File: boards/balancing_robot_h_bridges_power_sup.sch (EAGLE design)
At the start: 19 parts

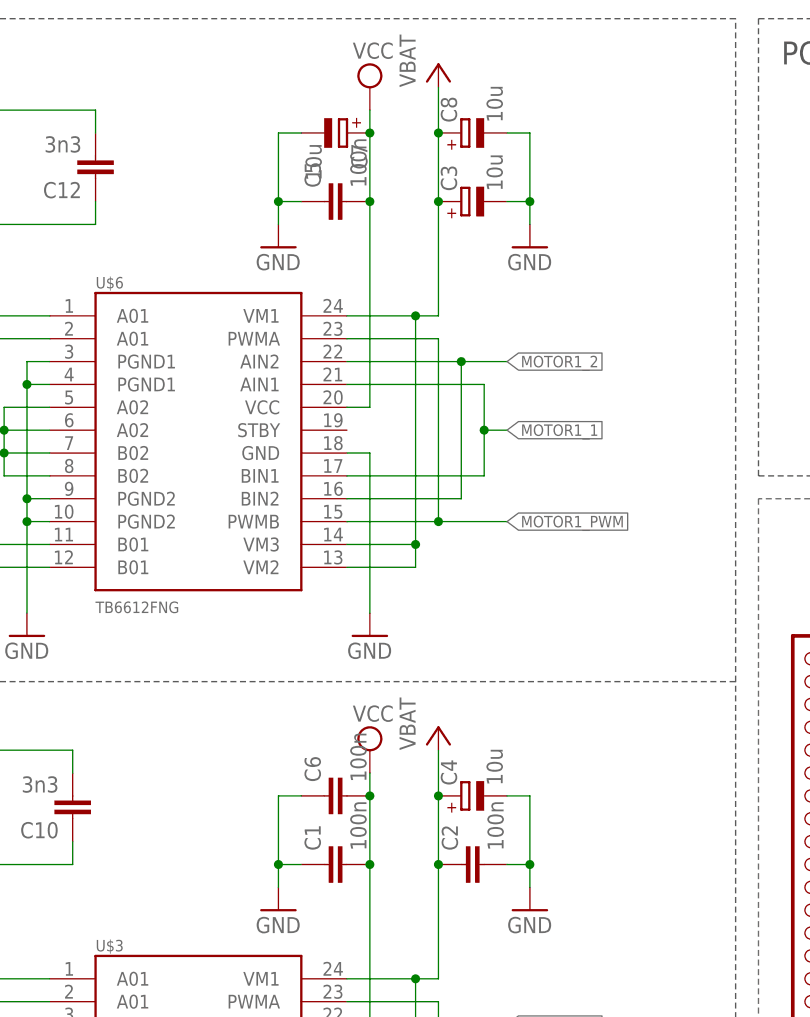
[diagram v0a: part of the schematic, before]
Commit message: updated bridge board
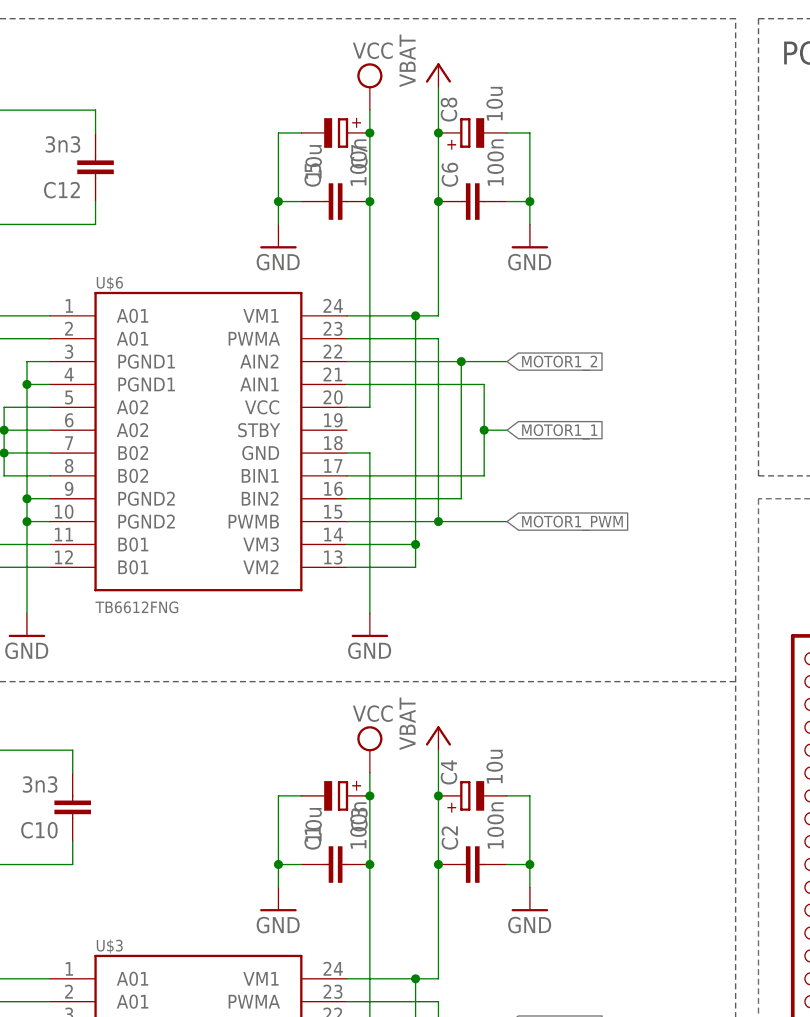
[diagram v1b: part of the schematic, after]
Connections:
- removed net N$5: U$3.PGND1@3, U$3.PGND1@4, U$3.PGND2@10, U$3.PGND2@9, U$6.PGND1@3, U$6.PGND1@4, U$6.PGND2@10, U$6.PGND2@9
- net GND: now also C6.2, U$3.PGND1@3, U$3.PGND1@4, U$3.PGND2@10, U$3.PGND2@9, U$6.PGND1@3, U$6.PGND1@4, U$6.PGND2@10, U$6.PGND2@9; no longer C6.1
- net VCC: now also C6.1; no longer C6.2
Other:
- moved on the sheet: C3, C6
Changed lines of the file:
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@@
 <part name="SUPPLY1" library="supply2" deviceset="VCC" device=""/>
 <part name="VAABT" library="supply1" deviceset="VCC" device="" value="VBAT"/>
-<part name="GND4" library="supply1" deviceset="GND" device=""/>
 <part name="GND5" library="supply1" deviceset="GND" device=""/>
 <part name="SUPPLY3" library="supply2" deviceset="VCC" device=""/>
@@
 <part name="GND7" library="supply1" deviceset="GND" device=""/>
 <part name="U$6" library="SparkFun-PowerIC" deviceset="TB6612FNG" device="" value="TB6612FNG"/>
-<part name="GND8" library="supply1" deviceset="GND" device=""/>
 <part name="GND9" library="supply1" deviceset="GND" device=""/>
 <part name="SUPPLY4" library="supply2" deviceset="VCC" device=""/>
-<part name="VAABT2" library="supply1" deviceset="VCC" device="" value="VBAT"/>
+<part name="VBAT" library="supply1" deviceset="VCC" device="" value="VBAT"/>
 <part name="C5" library="rcl" deviceset="C-EU" device="C0603" value="100n"/>
 <part name="GND10" library="supply1" deviceset="GND" device=""/>
@@
 <part name="C8" library="rcl" deviceset="CPOL-EU" device="153CLV-0405" value="10u"/>
 <part name="JP1" library="pinhead" deviceset="PINHD-1X24" device=""/>
-<part name="C3" library="rcl" deviceset="CPOL-EU" device="153CLV-0405" value="10u"/>
 <part name="C7" library="rcl" deviceset="CPOL-EU" device="153CLV-0405" value="10u"/>
-<part name="C6" library="rcl" deviceset="C-EU" device="C0603" value="100n"/>
 <part name="GND3" library="supply1" deviceset="GND" device=""/>
 <part name="VAABT3" library="supply1" deviceset="VCC" device="" value="VBAT"/>
+<part name="C3" library="rcl" deviceset="CPOL-EU" device="153CLV-0405" value="10u"/>
+<part name="C6" library="rcl" deviceset="C-EU" device="C0603" value="100n"/>
+<part name="GND8" library="supply1" deviceset="GND" device=""/>
+<part name="GND4" library="supply1" deviceset="GND" device=""/>
 </parts>
 <sheets>
@@
 <instance part="SUPPLY1" gate="G$1" x="195.58" y="134.62"/>
 <instance part="VAABT" gate="VCC" x="132.08" y="137.16"/>
-<instance part="GND4" gate="1" x="25.4" y="5.08"/>
 <instance part="GND5" gate="1" x="63.5" y="5.08"/>
 <instance part="SUPPLY3" gate="G$1" x="63.5" y="66.04"/>
@@
 <instance part="GND7" gate="1" x="81.28" y="48.26"/>
 <instance part="U$6" gate="G$1" x="45.72" y="101.6"/>
-<instance part="GND8" gate="1" x="25.4" y="78.74"/>
 <instance part="GND9" gate="1" x="63.5" y="78.74"/>
 <instance part="SUPPLY4" gate="G$1" x="63.5" y="139.7"/>
-<instance part="VAABT2" gate="VCC" x="71.12" y="142.24"/>
+<instance part="VBAT" gate="VCC" x="71.12" y="142.24"/>
 <instance part="C5" gate="G$1" x="58.42" y="127" rot="R90"/>
 <instance part="GND10" gate="1" x="53.34" y="121.92"/>
@@
 <instance part="C8" gate="G$1" x="73.66" y="134.62" rot="R90"/>
 <instance part="JP1" gate="A" x="111.76" y="45.72" rot="R180"/>
-<instance part="C3" gate="G$1" x="73.66" y="127" rot="R90"/>
 <instance part="C7" gate="G$1" x="60.96" y="134.62" rot="R270"/>
-<instance part="C6" gate="G$1" x="58.42" y="60.96" rot="R90"/>
 <instance part="GND3" gate="1" x="127" y="10.16"/>
 <instance part="VAABT3" gate="VCC" x="152.4" y="27.94"/>
+<instance part="C3" gate="G$1" x="60.96" y="60.96" rot="R270"/>
+<instance part="C6" gate="G$1" x="73.66" y="127" rot="R90"/>
+<instance part="GND8" gate="1" x="25.4" y="78.74"/>
+<instance part="GND4" gate="1" x="25.4" y="5.08"/>
 </instances>
 <busses>
@@
 <junction x="53.34" y="53.34"/>
 <pinref part="GND6" gate="1" pin="GND"/>
-<pinref part="C6" gate="G$1" pin="1"/>
+<pinref part="C3" gate="G$1" pin="-"/>
 </segment>
 <segment>
@@
 <pinref part="GND11" gate="1" pin="GND"/>
 <pinref part="C8" gate="G$1" pin="-"/>
-<pinref part="C3" gate="G$1" pin="-"/>
+<pinref part="C6" gate="G$1" pin="2"/>
 </segment>
 <segment>
@@
 <junction x="124.46" y="27.94"/>
 <pinref part="GND3" gate="1" pin="GND"/>
+</segment>
+<segment>
+<pinref part="U$6" gate="G$1" pin="PGND1@3"/>
+<wire x1="27.94" y1="109.22" x2="25.4" y2="109.22" width="0.1524" layer="91"/>
+<wire x1="25.4" y1="109.22" x2="25.4" y2="106.68" width="0.1524" layer="91"/>
+<pinref part="U$6" gate="G$1" pin="PGND2@10"/>
+<wire x1="25.4" y1="106.68" x2="25.4" y2="93.98" width="0.1524" layer="91"/>
+<wire x1="25.4" y1="93.98" x2="25.4" y2="91.44" width="0.1524" layer="91"/>
+<wire x1="25.4" y1="91.44" x2="25.4" y2="81.28" width="0.1524" layer="91"/>
+<wire x1="27.94" y1="91.44" x2="25.4" y2="91.44" width="0.1524" layer="91"/>
+<junction x="25.4" y="91.44"/>
+<pinref part="U$6" gate="G$1" pin="PGND2@9"/>
+<wire x1="27.94" y1="93.98" x2="25.4" y2="93.98" width="0.1524" layer="91"/>
+<junction x="25.4" y="93.98"/>
+<pinref part="U$6" gate="G$1" pin="PGND1@4"/>
+<wire x1="27.94" y1="106.68" x2="25.4" y2="106.68" width="0.1524" layer="91"/>
+<junction x="25.4" y="106.68"/>
+<pinref part="GND8" gate="1" pin="GND"/>
+</segment>
+<segment>
+<pinref part="U$3" gate="G$1" pin="PGND1@3"/>
+<wire x1="27.94" y1="35.56" x2="25.4" y2="35.56" width="0.1524" layer="91"/>
+<wire x1="25.4" y1="35.56" x2="25.4" y2="33.02" width="0.1524" layer="91"/>
+<pinref part="U$3" gate="G$1" pin="PGND2@10"/>
+<wire x1="25.4" y1="33.02" x2="25.4" y2="20.32" width="0.1524" layer="91"/>
+<wire x1="25.4" y1="20.32" x2="25.4" y2="17.78" width="0.1524" layer="91"/>
+<wire x1="25.4" y1="17.78" x2="25.4" y2="7.62" width="0.1524" layer="91"/>
+<wire x1="27.94" y1="17.78" x2="25.4" y2="17.78" width="0.1524" layer="91"/>
+<junction x="25.4" y="17.78"/>
+<pinref part="U$3" gate="G$1" pin="PGND2@9"/>
+<wire x1="27.94" y1="20.32" x2="25.4" y2="20.32" width="0.1524" layer="91"/>
+<junction x="25.4" y="20.32"/>
+<pinref part="U$3" gate="G$1" pin="PGND1@4"/>
+<wire x1="27.94" y1="33.02" x2="25.4" y2="33.02" width="0.1524" layer="91"/>
+<junction x="25.4" y="33.02"/>
+<pinref part="GND4" gate="1" pin="GND"/>
 </segment>
 </net>
@@
 <wire x1="63.5" y1="53.34" x2="63.5" y2="60.96" width="0.1524" layer="91"/>
 <junction x="63.5" y="53.34"/>
-<pinref part="C6" gate="G$1" pin="2"/>
+<pinref part="C3" gate="G$1" pin="+"/>
 <wire x1="63.5" y1="60.96" x2="63.5" y2="63.5" width="0.1524" layer="91"/>
 <junction x="63.5" y="60.96"/>
@@
 <wire x1="60.96" y1="88.9" x2="68.58" y2="88.9" width="0.1524" layer="91"/>
 <junction x="68.58" y="88.9"/>
-<pinref part="VAABT2" gate="VCC" pin="VCC"/>
+<pinref part="VBAT" gate="VCC" pin="VCC"/>
 <wire x1="68.58" y1="114.3" x2="71.12" y2="114.3" width="0.1524" layer="91"/>
 <wire x1="71.12" y1="114.3" x2="71.12" y2="127" width="0.1524" layer="91"/>
@@
 <wire x1="71.12" y1="134.62" x2="71.12" y2="139.7" width="0.1524" layer="91"/>
 <junction x="71.12" y="134.62"/>
-<pinref part="C3" gate="G$1" pin="+"/>
+<pinref part="C6" gate="G$1" pin="1"/>
 <junction x="71.12" y="127"/>
 </segment>
@@
 </segment>
 </net>
-<net name="N$5" class="0">
-<segment>
-<pinref part="U$3" gate="G$1" pin="PGND1@3"/>
-<wire x1="27.94" y1="35.56" x2="25.4" y2="35.56" width="0.1524" layer="91"/>
-<wire x1="25.4" y1="35.56" x2="25.4" y2="33.02" width="0.1524" layer="91"/>
-<pinref part="U$3" gate="G$1" pin="PGND2@10"/>
-<wire x1="25.4" y1="33.02" x2="25.4" y2="20.32" width="0.1524" layer="91"/>
-<wire x1="25.4" y1="20.32" x2="25.4" y2="17.78" width="0.1524" layer="91"/>
-<wire x1="25.4" y1="17.78" x2="25.4" y2="7.62" width="0.1524" layer="91"/>
-<wire x1="27.94" y1="17.78" x2="25.4" y2="17.78" width="0.1524" layer="91"/>
-<junction x="25.4" y="17.78"/>
-<pinref part="U$3" gate="G$1" pin="PGND2@9"/>
-<wire x1="27.94" y1="20.32" x2="25.4" y2="20.32" width="0.1524" layer="91"/>
-<junction x="25.4" y="20.32"/>
-<pinref part="U$3" gate="G$1" pin="PGND1@4"/>
-<wire x1="27.94" y1="33.02" x2="25.4" y2="33.02" width="0.1524" layer="91"/>
-<junction x="25.4" y="33.02"/>
-<pinref part="GND4" gate="1" pin="GND"/>
-</segment>
-<segment>
-<pinref part="U$6" gate="G$1" pin="PGND1@3"/>
-<wire x1="27.94" y1="109.22" x2="25.4" y2="109.22" width="0.1524" layer="91"/>
-<wire x1="25.4" y1="109.22" x2="25.4" y2="106.68" width="0.1524" layer="91"/>
-<pinref part="U$6" gate="G$1" pin="PGND2@10"/>
-<wire x1="25.4" y1="106.68" x2="25.4" y2="93.98" width="0.1524" layer="91"/>
-<wire x1="25.4" y1="93.98" x2="25.4" y2="91.44" width="0.1524" layer="91"/>
-<wire x1="25.4" y1="91.44" x2="25.4" y2="81.28" width="0.1524" layer="91"/>
-<wire x1="27.94" y1="91.44" x2="25.4" y2="91.44" width="0.1524" layer="91"/>
-<junction x="25.4" y="91.44"/>
-<pinref part="U$6" gate="G$1" pin="PGND2@9"/>
-<wire x1="27.94" y1="93.98" x2="25.4" y2="93.98" width="0.1524" layer="91"/>
-<junction x="25.4" y="93.98"/>
-<pinref part="U$6" gate="G$1" pin="PGND1@4"/>
-<wire x1="27.94" y1="106.68" x2="25.4" y2="106.68" width="0.1524" layer="91"/>
-<junction x="25.4" y="106.68"/>
-<pinref part="GND8" gate="1" pin="GND"/>
-</segment>
-</net>
